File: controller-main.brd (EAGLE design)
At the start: 91.1 x 80 mm, 26 parts

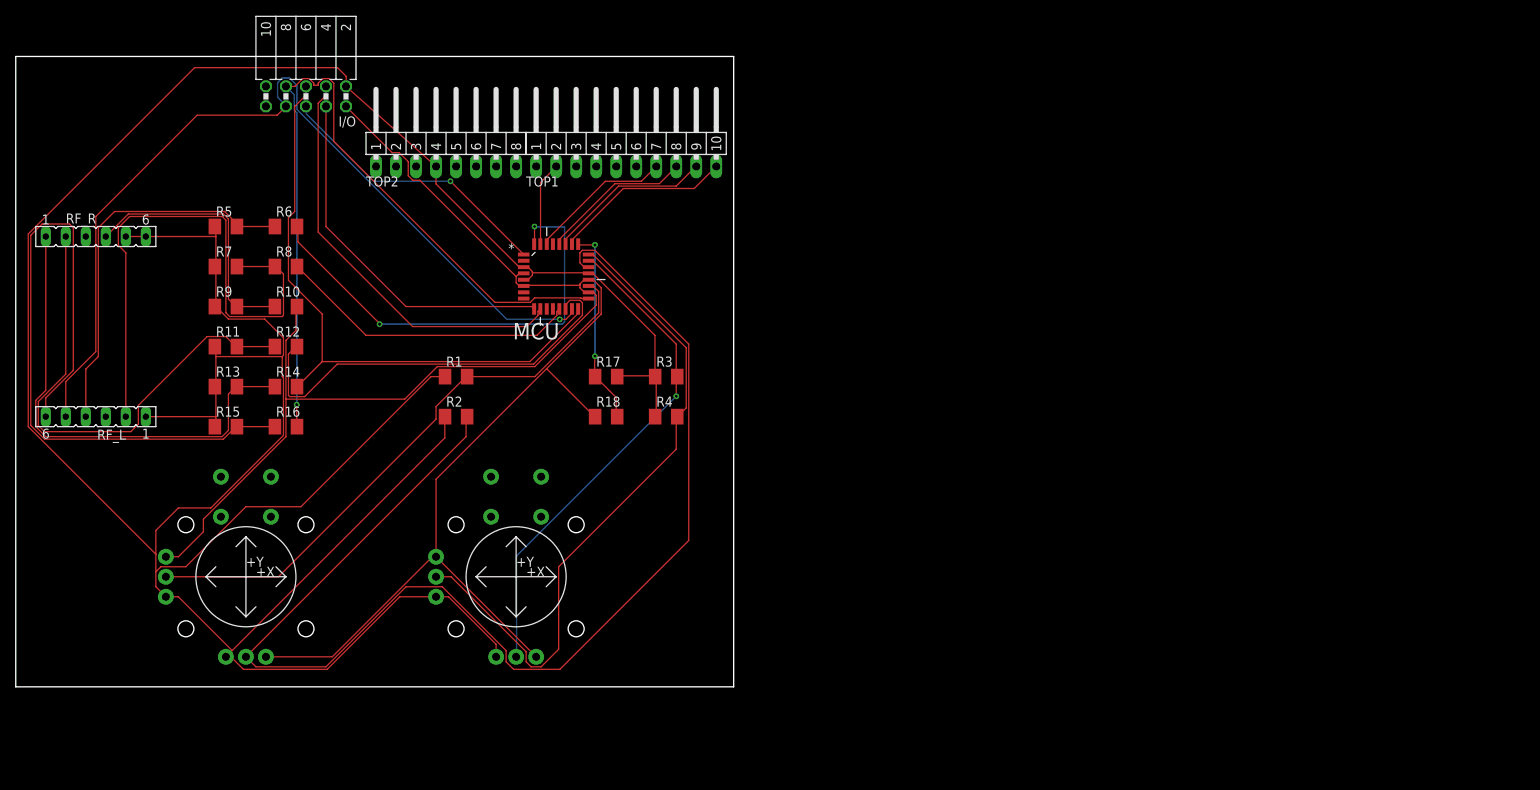
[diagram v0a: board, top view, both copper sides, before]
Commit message: only half done
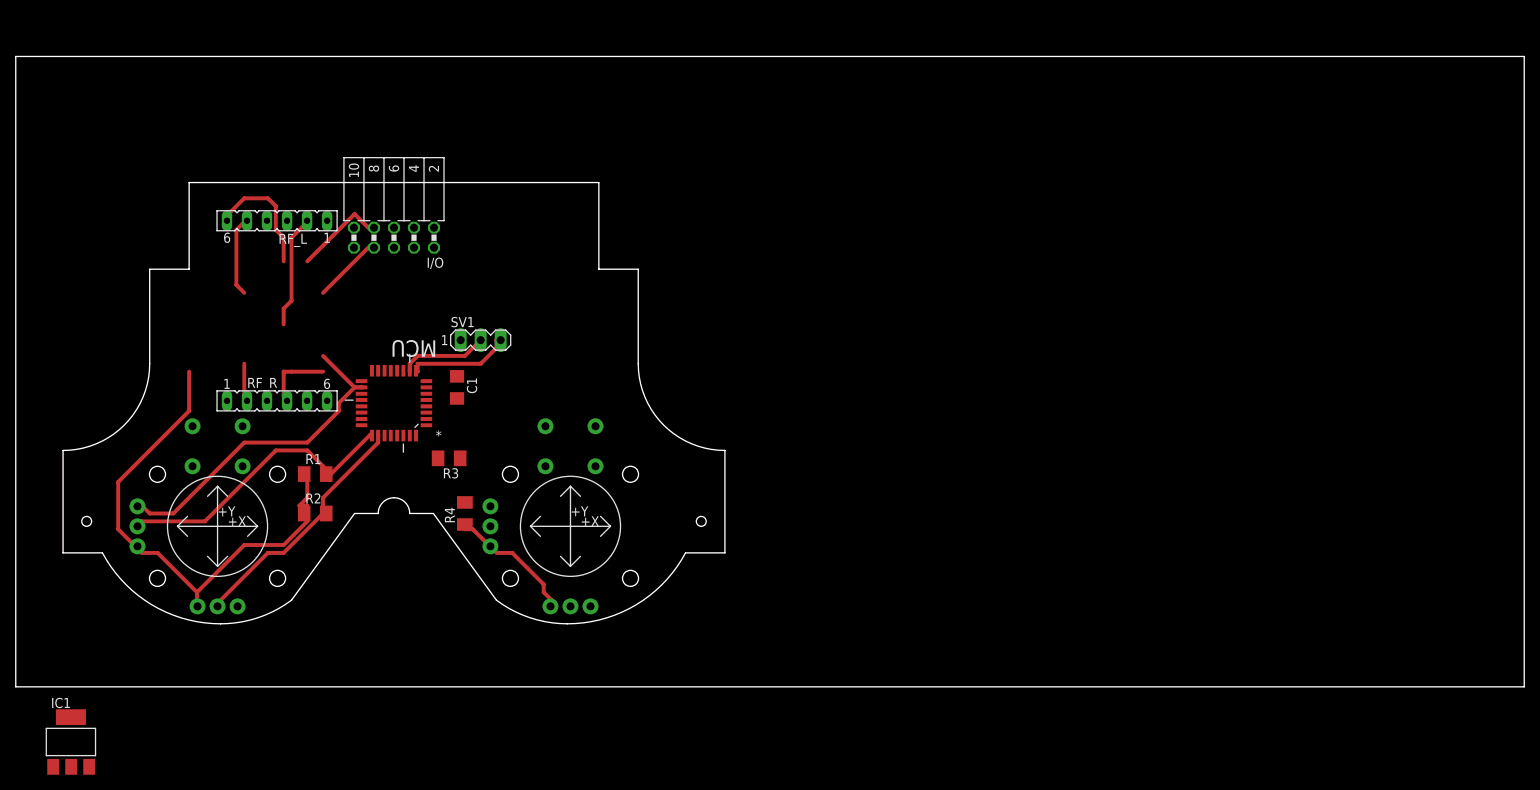
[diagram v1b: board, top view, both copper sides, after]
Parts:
- removed R10, R12, R14, R16, R17, R18, R6, R8: 1k, resistor:M1206
- removed R11, R13, R15, R5, R7, R9: 2k, resistor:M1206
- removed TOP1: (no value), con-lstb:MA10-1W
- removed TOP2: (no value), con-lstb:MA08-1W
- added C1: (no value), resistor:C1206
- added IC1: REG1117, burr-brown:SOT223
- added SV1: (no value), con-lstb:MA03-1
- moved RF_L 33.9 mm to (33.2, 59.1)
- moved RF_R 31.1 mm to (33.2, 36.3)
- moved R3 29.4 mm to (55.0, 29.0), turned to 180 degrees
- moved R4 28.4 mm to (57.0, 22.0), turned to 90 degrees
- moved MCU 26.1 mm to (48.0, 36.0), turned to 180 degrees
- moved R1 21.7 mm to (38.0, 27.0)
- moved R2 21.7 mm to (38.0, 22.0)
- moved I/O 21.1 mm to (48.0, 57.0)
- moved RAN 9.41 mm to (70.4, 20.4)
- moved LAN 7.34 mm to (25.6, 20.4)
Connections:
- removed net 4D_INT: I/O.5, MCU.1
- removed net BATP: MCU.25, R17.1, R18.2
- removed net BL: MCU.27, TOP1.9
- removed net BR: MCU.28, TOP1.8
- removed net BU: MCU.26, TOP1.10
- removed net MISO_LOW: R13.2, R14.1, RF_R.1
- removed net RF_CS_LOW: R11.2, R12.1, RF_R.2
- removed net RF_INT_LOW: R5.2, R6.1, RF_L.4
- removed net RF_RES_LOW: R7.2, R8.1, RF_L.2
- removed net SCK_LOW: R15.2, R16.1, RF_L.6
- net 3.3V: now also IC1.2; no longer R10.1, R9.2
- net 4D_CS: now also I/O.5, MCU.12; no longer I/O.4, MCU.10
- net 4D_PD: now also MCU.11; no longer MCU.9
- net 5V: now also C1.1, IC1.3; no longer R10.2, R18.1
- net BD: now also MCU.9, SV1.3; no longer MCU.30, TOP1.7
- net GND: now also C1.2, IC1.1, SV1.1; no longer R11.1, R13.1, R15.1, R17.2, R5.1, R7.1, R9.1, TOP2.4
- net LAX: now also MCU.26; no longer MCU.22
- net LAY: now also MCU.25; no longer MCU.19
- net MISO: now also RF_R.1; no longer R14.2
- net RAX: now also MCU.28; no longer MCU.23
- net RAY: now also MCU.27; no longer MCU.24
- net RF_CS: now also RF_R.2; no longer R12.2
- net RF_INT: now also MCU.1, RF_L.4; no longer MCU.32, R6.2
- net RF_RES: now also RF_L.2; no longer R8.2
- net SCK: now also RF_L.6; no longer R16.2
- net SEL: now also MCU.10, SV1.2; no longer MCU.31, TOP1.2
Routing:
- net GND: track 414.3 -> 80.4 mm
- net 5V: track 230.0 -> 42.0 mm
- net LAX: track 161.4 -> 31.9 mm
- net MOSI: track 113.3 -> 19.2 mm, vias 1 -> 0
- net SCK_LOW: track 88.1 -> 0.00 mm
- net RAY: track 84.4 -> 0.00 mm
- net MISO: track 77.8 -> 0.00 mm
- net SCK: track 99.9 -> 27.4 mm, vias 1 -> 0
- net RF_RES_LOW: track 69.7 -> 0.00 mm
- net RAX: track 63.9 -> 0.00 mm, vias 1 -> 0
- net RF_CS_LOW: track 62.7 -> 0.00 mm
- net MISO_LOW: track 60.9 -> 0.00 mm
- net RF_INT: track 58.7 -> 0.00 mm, vias 2 -> 0
- net 4D_CS: track 54.0 -> 0.00 mm
- net RF_INT_LOW: track 49.1 -> 0.00 mm
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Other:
- board size 91.1 x 80 mm -> 191.4 x 80 mm

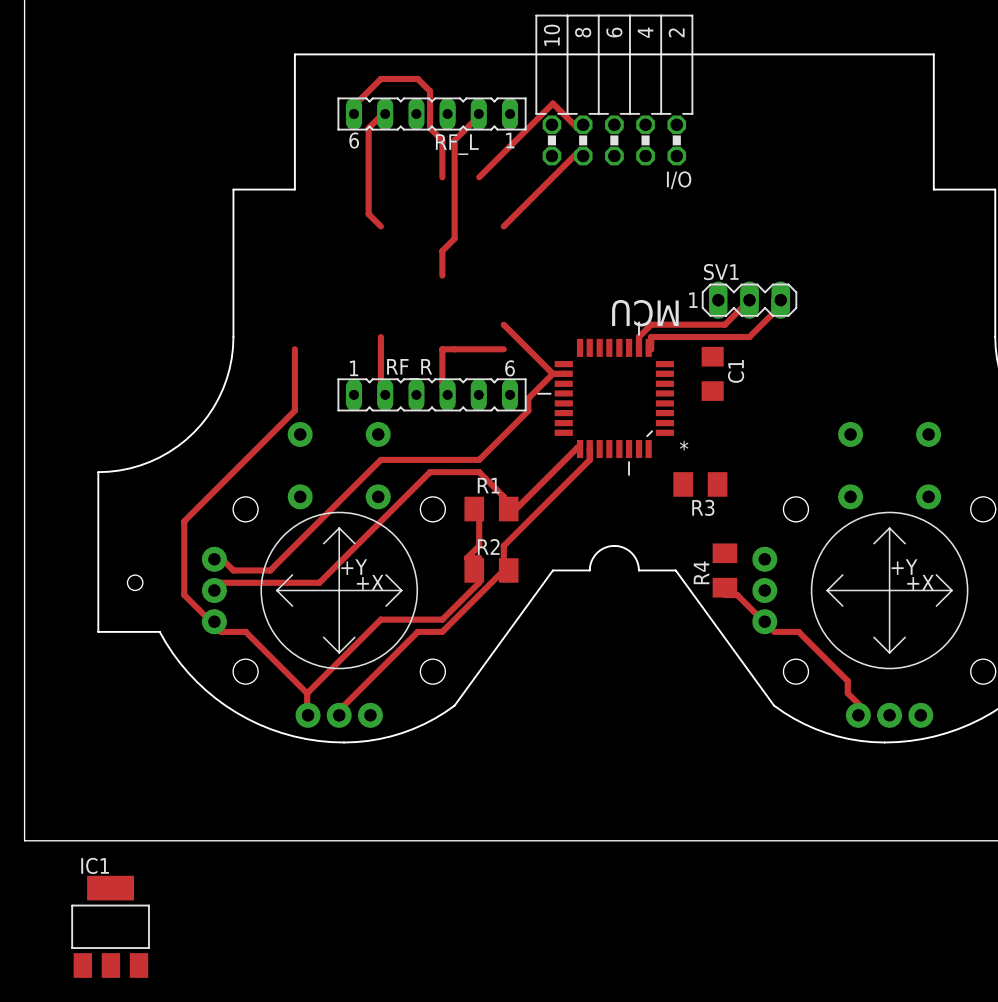
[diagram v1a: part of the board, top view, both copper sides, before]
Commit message: finished the main board
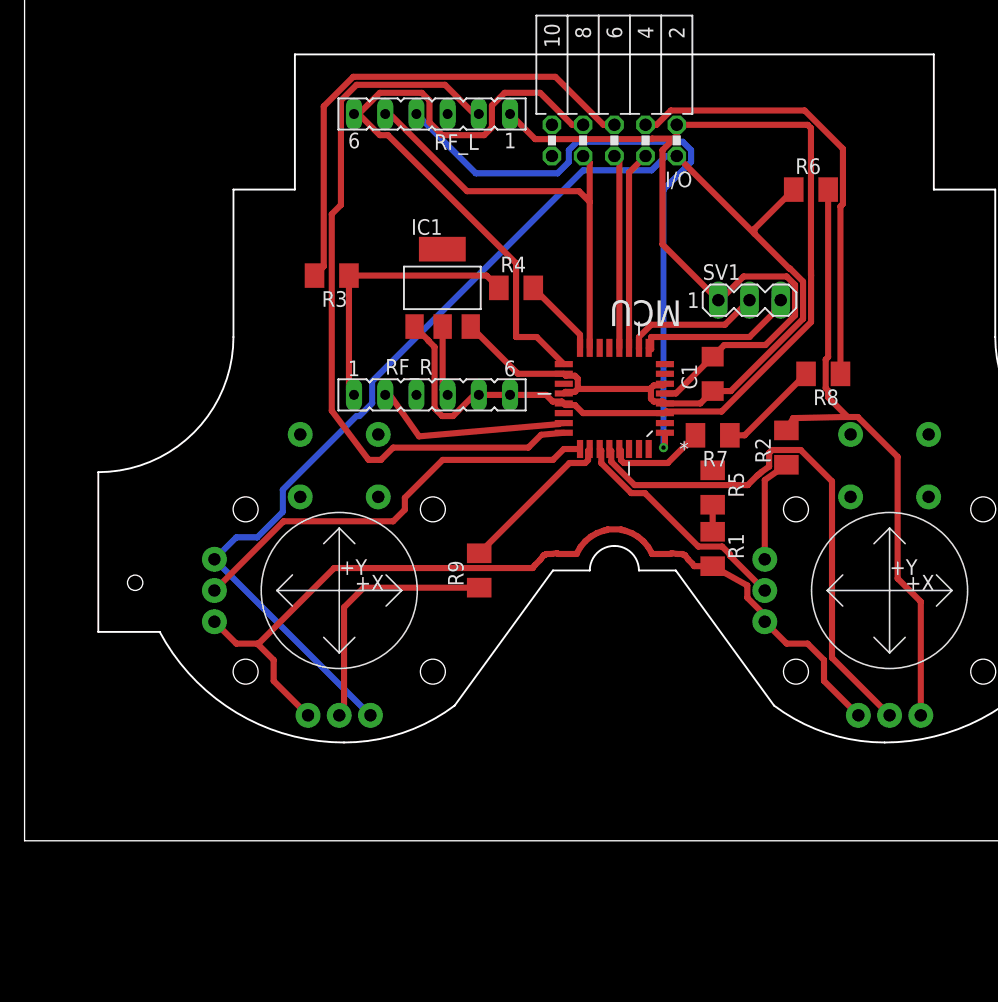
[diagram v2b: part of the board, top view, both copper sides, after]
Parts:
- added R5, R6, R7, R8, R9: (no value), resistor:M1206
- R1, R2, R3, R4: value 10k -> (none)
- moved IC1 58.6 mm to (34.0, 45.0)
- moved R3 34.5 mm to (25.0, 46.0)
- moved R4 28.6 mm to (40.0, 45.0), turned to 0 degrees
- moved R2 26.0 mm to (62.0, 32.0), turned to 90 degrees
- moved R1 18.3 mm to (56.0, 23.8), turned to 270 degrees
- turned C1 to 90 degrees
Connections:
- new net 5V2: R2.2, R6.2, RAN.VCCX
- new net 5V_R: R2.1, RAN.VCCY
- new net GND_R: LAN.GNDX, LAN.GNDY, R1.2, RAN.GNDX, RAN.GNDY
- new net MISO2: I/O.6, R3.2
- new net MISO3: MCU.16, R4.2
- new net N$1: R1.1, R5.2
- new net N$2: LAN.OUTX, R9.1
- new net RST: MCU.29, R7.2
- new net RST2: R7.1, R8.2
- new net RST3: I/O.4, R8.1
- net 5V: now also R6.1; no longer RAN.VCCX, RAN.VCCY
- net GND: now also R5.1; no longer LAN.GNDX, LAN.GNDY, R1.1, R2.1, R3.1, R4.1, RAN.GNDX, RAN.GNDY
- net LAX: now also R9.2; no longer LAN.OUTX, R2.2
- net LAY: no longer R1.2
- net MISO: now also R3.1, R4.1; no longer I/O.6, MCU.16
- net RAX: no longer R3.2
- net RAY: no longer R4.2
- net RF_CS: now also MCU.23; no longer MCU.14
- net RF_RES: now also MCU.24; no longer MCU.13
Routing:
- net 5V: track 42.0 -> 129.8 mm
- net GND_R: track 0.00 -> 72.6 mm
- net RF_INT: track 0.00 -> 52.7 mm, vias 0 -> 1
- net 5V2: track 0.00 -> 52.1 mm
- net RF_RES: track 14.4 -> 60.0 mm
- net RAX: track 0.00 -> 43.7 mm
- net GND: track 80.4 -> 123.8 mm
- net MISO2: track 0.00 -> 40.4 mm
- net RST3: track 0.00 -> 36.2 mm
- net SCK: track 27.4 -> 54.4 mm
- net MISO: track 0.00 -> 22.5 mm
- net N$2: track 0.00 -> 20.6 mm
- net LAX: track 31.9 -> 13.0 mm
- net RAY: track 0.00 -> 18.9 mm
- net MOSI: track 19.2 -> 35.4 mm
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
